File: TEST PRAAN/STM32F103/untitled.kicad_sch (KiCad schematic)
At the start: 18 parts

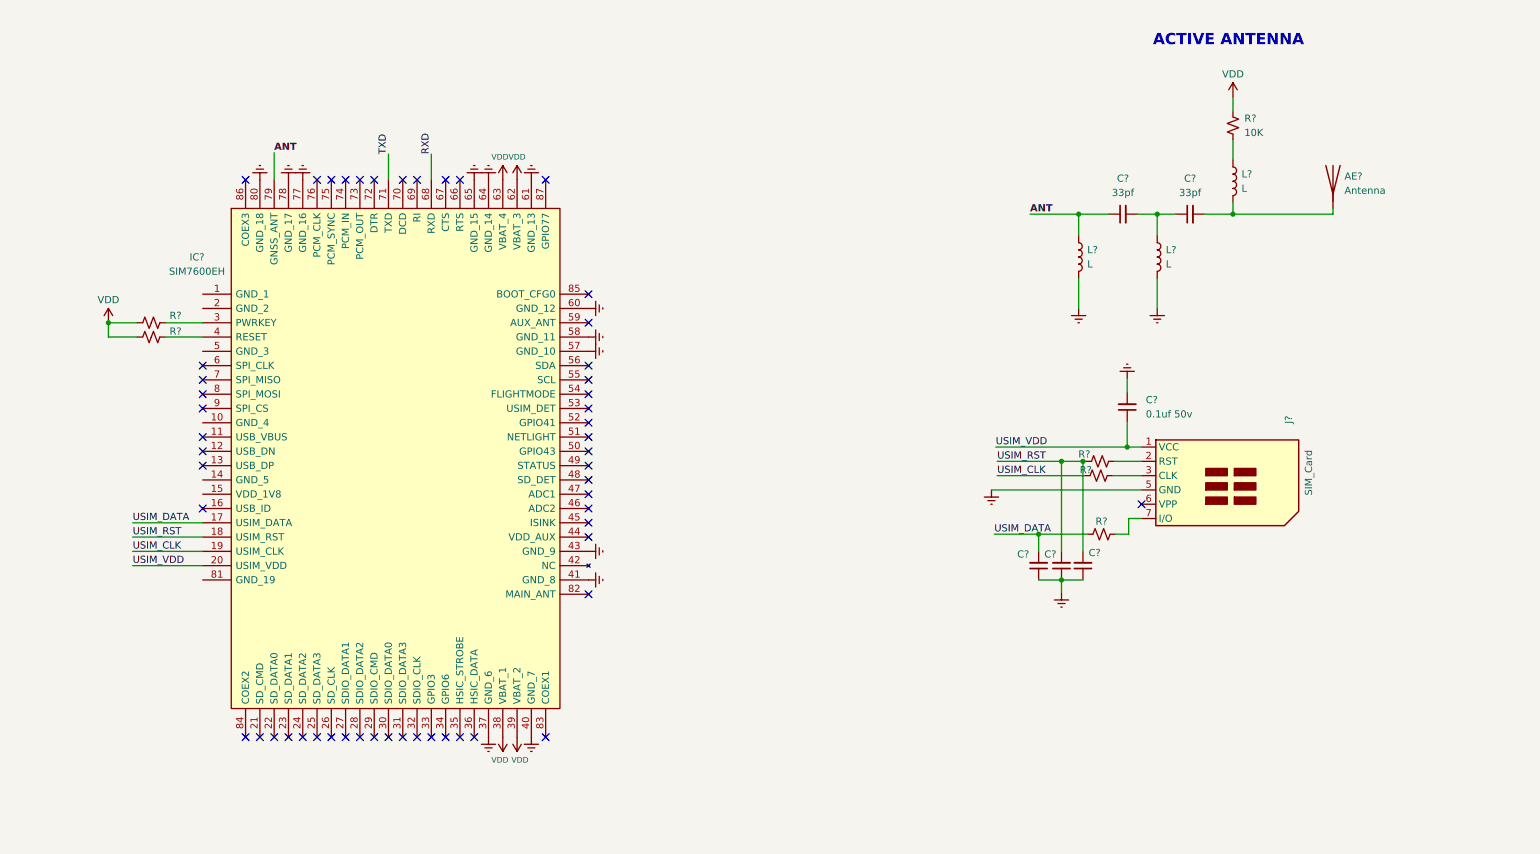
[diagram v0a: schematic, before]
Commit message: UPDATE
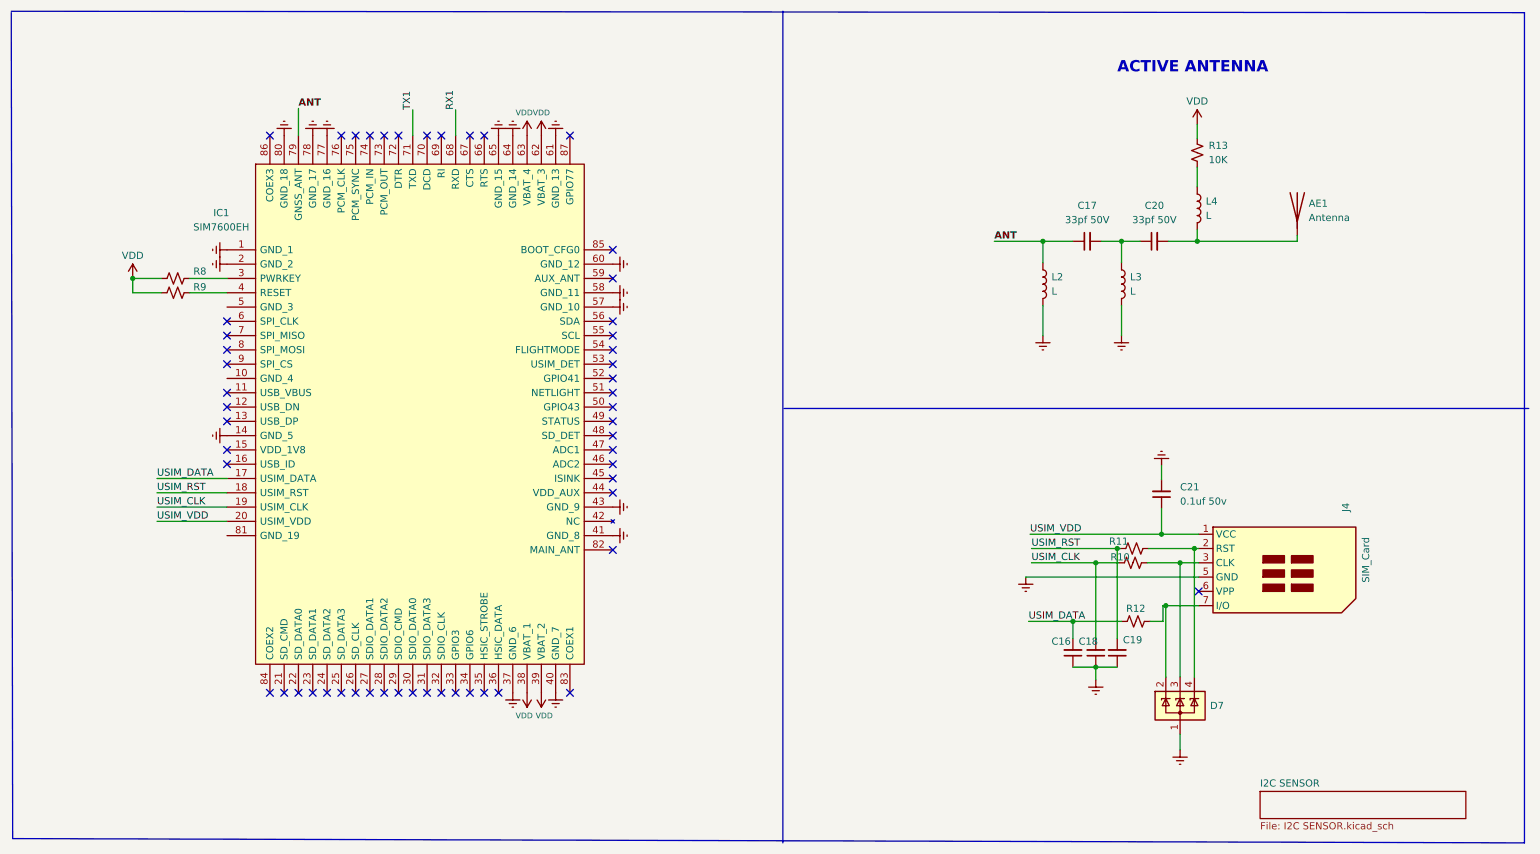
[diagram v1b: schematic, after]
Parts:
- added D7: SP0503BAHT, Package_TO_SOT_SMD:SOT-143, symbol Power_Protection:SP0503BAHT
- AE1: renamed from AE?; footprint (none) -> RF_Antenna:Texas_SWRA117D_2.4GHz_Right
- C16, C18, C19, C21: renamed from C?; footprint (none) -> Capacitor_SMD:C_0805_2012Metric_Pad1.18x1.45mm_HandSolder
- C17, C20: renamed from C?; value 33pf -> 33pf 50V; footprint (none) -> Capacitor_SMD:C_0805_2012Metric_Pad1.18x1.45mm_HandSolder
- IC1: renamed from IC?; footprint SIM7600EH -> Library:SIM7600EH
- J4: renamed from J?; footprint (none) -> Connector_Card:microSIM_JAE_SF53S006VCBR2000
- L2, L3, L4: renamed from L?; footprint (none) -> Inductor_SMD:L_1206_3216Metric_Pad1.42x1.75mm_HandSolder
- R10, R11, R12, R13, R8, R9: renamed from R?; footprint (none) -> Resistor_SMD:R_0805_2012Metric_Pad1.20x1.40mm_HandSolder
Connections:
- net Earth: now also IC1.1 (GND_1), IC1.14 (GND_5), IC1.2 (GND_2), D7.1 (A)
- net USIM_CLK: now also C18.2
- net USIM_RST: no longer C18.2
- net at J4.2 (RST), R11.2: now also D7.4 (K)
- net at J4.3 (CLK), R10.2: now also D7.3 (K)
- net at J4.7 (I/O), R12.2: now also D7.2 (K)
- net RXD renamed RX1
- net TXD renamed TX1
- no-connect marks 54 -> 55
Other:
- added sheet I2C SENSOR (I2C SENSOR.kicad_sch)
- moved on the sheet: AE1, C16, C17, C18, C19, C20, C21, IC1, J4, L2, L3, L4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
